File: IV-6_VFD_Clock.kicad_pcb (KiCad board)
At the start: 2 copper layers, 162 x 52 mm, 0 parts

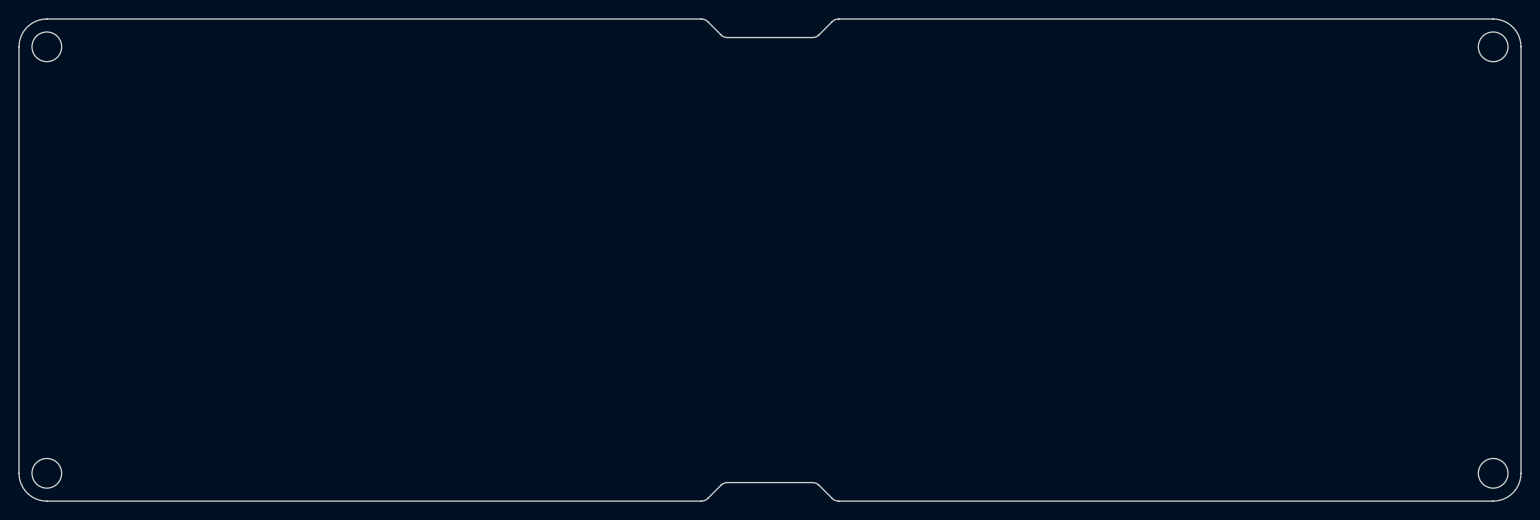
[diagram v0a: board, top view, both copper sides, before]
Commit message: PSU Design started
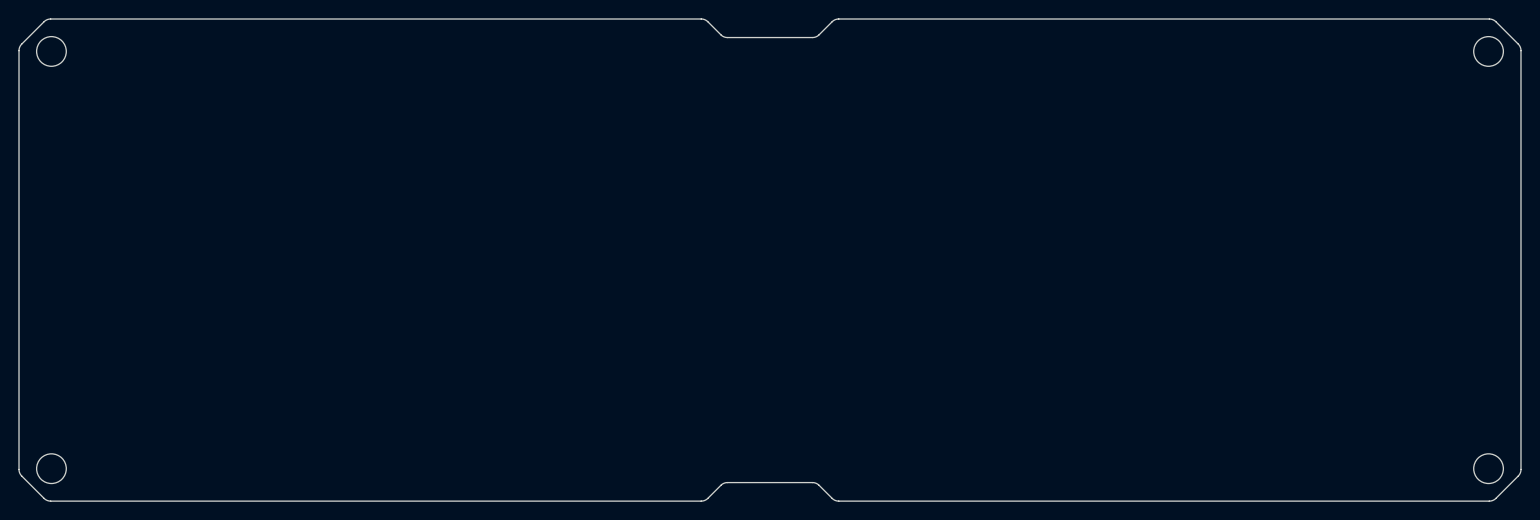
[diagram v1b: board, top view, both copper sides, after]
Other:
- outline, holes or cut-outs redrawn
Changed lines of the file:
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@@
 	)
 	(net 0 "")
-	(gr_arc
-		(start 33 82)
-		(mid 30.87868 81.12132)
-		(end 30 79)
-		(stroke
-			(width 0.1)
-			(type default)
-		)
-		(layer "Edge.Cuts")
-	)
-	(gr_line
-		(start 30 79)
-		(end 30 33)
+	(gr_line
+		(start 30 78.585786)
+		(end 30 33.414214)
 		(stroke
 			(width 0.1)
@@
 	(gr_line
 		(start 118.414214 30)
-		(end 189 30)
+		(end 188.585786 30)
+		(stroke
+			(width 0.1)
+			(type default)
+		)
+		(layer "Edge.Cuts")
+	)
+	(gr_arc
+		(start 192 78.585786)
+		(mid 191.923884 78.968472)
+		(end 191.707107 79.292893)
+		(stroke
+			(width 0.1)
+			(type default)
+		)
+		(layer "Edge.Cuts")
+	)
+	(gr_arc
+		(start 189.292893 81.707107)
+		(mid 188.96847 81.92388)
+		(end 188.585786 82)
 		(stroke
 			(width 0.1)
@@
 	(gr_line
 		(start 103.585786 82)
-		(end 33 82)
+		(end 33.414214 82)
 		(stroke
 			(width 0.1)
@@
 	)
 	(gr_circle
-		(center 189 33)
-		(end 190.6 33)
+		(center 188.5 33.5)
+		(end 190.1 33.5)
 		(stroke
 			(width 0.1)
@@
 		)
 		(fill no)
+		(layer "Edge.Cuts")
+	)
+	(gr_arc
+		(start 106.414214 32)
+		(mid 106.031528 31.923884)
+		(end 105.707107 31.707107)
+		(stroke
+			(width 0.1)
+			(type default)
+		)
 		(layer "Edge.Cuts")
 	)
@@
 	)
 	(gr_arc
-		(start 117.707107 30.292893)
-		(mid 118.03153 30.07612)
-		(end 118.414214 30)
-		(stroke
-			(width 0.1)
-			(type default)
-		)
-		(layer "Edge.Cuts")
-	)
-	(gr_arc
-		(start 30 33)
-		(mid 30.87868 30.87868)
-		(end 33 30)
-		(stroke
-			(width 0.1)
-			(type default)
-		)
-		(layer "Edge.Cuts")
-	)
-	(gr_arc
-		(start 118.414214 82)
-		(mid 118.031528 81.923884)
-		(end 117.707107 81.707107)
-		(stroke
-			(width 0.1)
-			(type default)
-		)
-		(layer "Edge.Cuts")
-	)
-	(gr_line
-		(start 33 30)
+		(start 116.292893 31.707107)
+		(mid 115.968469 31.923875)
+		(end 115.585786 32)
+		(stroke
+			(width 0.1)
+			(type default)
+		)
+		(layer "Edge.Cuts")
+	)
+	(gr_line
+		(start 33.414214 30)
 		(end 103.585786 30)
 		(stroke
 			(width 0.1)
+			(type solid)
+		)
+		(layer "Edge.Cuts")
+	)
+	(gr_line
+		(start 189.292893 81.707107)
+		(end 191.707107 79.292893)
+		(stroke
+			(width 0.1)
 			(type default)
 		)
@@
 	)
 	(gr_circle
-		(center 189 79)
-		(end 190.6 79)
+		(center 188.5 78.5)
+		(end 190.1 78.5)
 		(stroke
 			(width 0.1)
@@
 	)
 	(gr_arc
-		(start 103.585786 30)
-		(mid 103.968469 30.07612)
-		(end 104.292893 30.292893)
+		(start 188.585786 30)
+		(mid 188.968469 30.07612)
+		(end 189.292893 30.292893)
 		(stroke
 			(width 0.1)
@@
 		(start 106.414214 80)
 		(end 115.585786 80)
+		(stroke
+			(width 0.1)
+			(type default)
+		)
+		(layer "Edge.Cuts")
+	)
+	(gr_arc
+		(start 104.292893 81.707107)
+		(mid 103.968469 81.923875)
+		(end 103.585786 82)
+		(stroke
+			(width 0.1)
+			(type default)
+		)
+		(layer "Edge.Cuts")
+	)
+	(gr_circle
+		(center 33.5 78.5)
+		(end 35.1 78.5)
+		(stroke
+			(width 0.1)
+			(type solid)
+		)
+		(fill no)
+		(layer "Edge.Cuts")
+	)
+	(gr_line
+		(start 30.292893 79.292893)
+		(end 32.707107 81.707107)
+		(stroke
+			(width 0.1)
+			(type default)
+		)
+		(layer "Edge.Cuts")
+	)
+	(gr_arc
+		(start 118.414214 82)
+		(mid 118.031531 81.92388)
+		(end 117.707107 81.707107)
+		(stroke
+			(width 0.1)
+			(type default)
+		)
+		(layer "Edge.Cuts")
+	)
+	(gr_arc
+		(start 30 33.414214)
+		(mid 30.076116 33.031528)
+		(end 30.292893 32.707107)
+		(stroke
+			(width 0.1)
+			(type default)
+		)
+		(layer "Edge.Cuts")
+	)
+	(gr_arc
+		(start 117.707107 30.292893)
+		(mid 118.031531 30.076125)
+		(end 118.414214 30)
+		(stroke
+			(width 0.1)
+			(type default)
+		)
+		(layer "Edge.Cuts")
+	)
+	(gr_line
+		(start 30.292893 32.707107)
+		(end 32.707107 30.292893)
+		(stroke
+			(width 0.1)
+			(type default)
+		)
+		(layer "Edge.Cuts")
+	)
+	(gr_line
+		(start 188.585786 82)
+		(end 118.414214 82)
+		(stroke
+			(width 0.1)
+			(type default)
+		)
+		(layer "Edge.Cuts")
+	)
+	(gr_arc
+		(start 105.707107 80.292893)
+		(mid 106.03153 80.07612)
+		(end 106.414214 80)
+		(stroke
+			(width 0.1)
+			(type default)
+		)
+		(layer "Edge.Cuts")
+	)
+	(gr_arc
+		(start 191.707107 32.707107)
+		(mid 191.923875 33.031531)
+		(end 192 33.414214)
+		(stroke
+			(width 0.1)
+			(type default)
+		)
+		(layer "Edge.Cuts")
+	)
+	(gr_line
+		(start 192 33.414214)
+		(end 192 78.585786)
+		(stroke
+			(width 0.1)
+			(type default)
+		)
+		(layer "Edge.Cuts")
+	)
+	(gr_arc
+		(start 30.292893 79.292893)
+		(mid 30.076125 78.968469)
+		(end 30 78.585786)
 		(stroke
 			(width 0.1)
@@
 		(layer "Edge.Cuts")
 	)
-	(gr_arc
-		(start 106.414214 32)
-		(mid 106.031531 31.92388)
-		(end 105.707107 31.707107)
-		(stroke
-			(width 0.1)
-			(type default)
-		)
-		(layer "Edge.Cuts")
-	)
 	(gr_circle
-		(center 33 79)
-		(end 34.6 79)
-		(stroke
-			(width 0.1)
-			(type solid)
-		)
-		(fill no)
-		(layer "Edge.Cuts")
-	)
-	(gr_arc
-		(start 105.707107 80.292893)
-		(mid 106.031531 80.076125)
-		(end 106.414214 80)
-		(stroke
-			(width 0.1)
-			(type default)
-		)
-		(layer "Edge.Cuts")
-	)
-	(gr_line
-		(start 189 82)
-		(end 118.414214 82)
-		(stroke
-			(width 0.1)
-			(type default)
-		)
-		(layer "Edge.Cuts")
-	)
-	(gr_line
-		(start 192 33)
-		(end 192 79)
-		(stroke
-			(width 0.1)
-			(type default)
-		)
-		(layer "Edge.Cuts")
-	)
-	(gr_arc
-		(start 116.292893 31.707107)
-		(mid 115.968469 31.923875)
-		(end 115.585786 32)
-		(stroke
-			(width 0.1)
-			(type default)
-		)
-		(layer "Edge.Cuts")
-	)
-	(gr_circle
-		(center 33 33)
-		(end 34.6 33)
+		(center 33.5 33.5)
+		(end 35.1 33.5)
 		(stroke
 			(width 0.1)
@@
 		(layer "Edge.Cuts")
 	)
-	(gr_arc
-		(start 189 30)
-		(mid 191.12132 30.87868)
-		(end 192 33)
-		(stroke
-			(width 0.1)
-			(type default)
-		)
-		(layer "Edge.Cuts")
-	)
 	(gr_line
 		(start 105.707107 80.292893)
@@
 	)
 	(gr_arc
-		(start 192 79)
-		(mid 191.12132 81.12132)
-		(end 189 82)
-		(stroke
-			(width 0.1)
-			(type default)
-		)
-		(layer "Edge.Cuts")
-	)
-	(gr_arc
-		(start 104.292893 81.707107)
-		(mid 103.96847 81.92388)
-		(end 103.585786 82)
+		(start 32.707107 30.292893)
+		(mid 33.03153 30.07612)
+		(end 33.414214 30)
+		(stroke
+			(width 0.1)
+			(type default)
+		)
+		(layer "Edge.Cuts")
+	)
+	(gr_arc
+		(start 33.414214 82)
+		(mid 33.031531 81.92388)
+		(end 32.707107 81.707107)
+		(stroke
+			(width 0.1)
+			(type default)
+		)
+		(layer "Edge.Cuts")
+	)
+	(gr_arc
+		(start 103.585786 30)
+		(mid 103.968472 30.076116)
+		(end 104.292893 30.292893)
 		(stroke
 			(width 0.1)
@@
 		(stroke
 			(width 0.1)
+			(type default)
+		)
+		(layer "Edge.Cuts")
+	)
+	(gr_line
+		(start 189.292893 30.292893)
+		(end 191.707107 32.707107)
+		(stroke
+			(width 0.1)
